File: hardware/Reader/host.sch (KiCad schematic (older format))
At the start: 7 parts

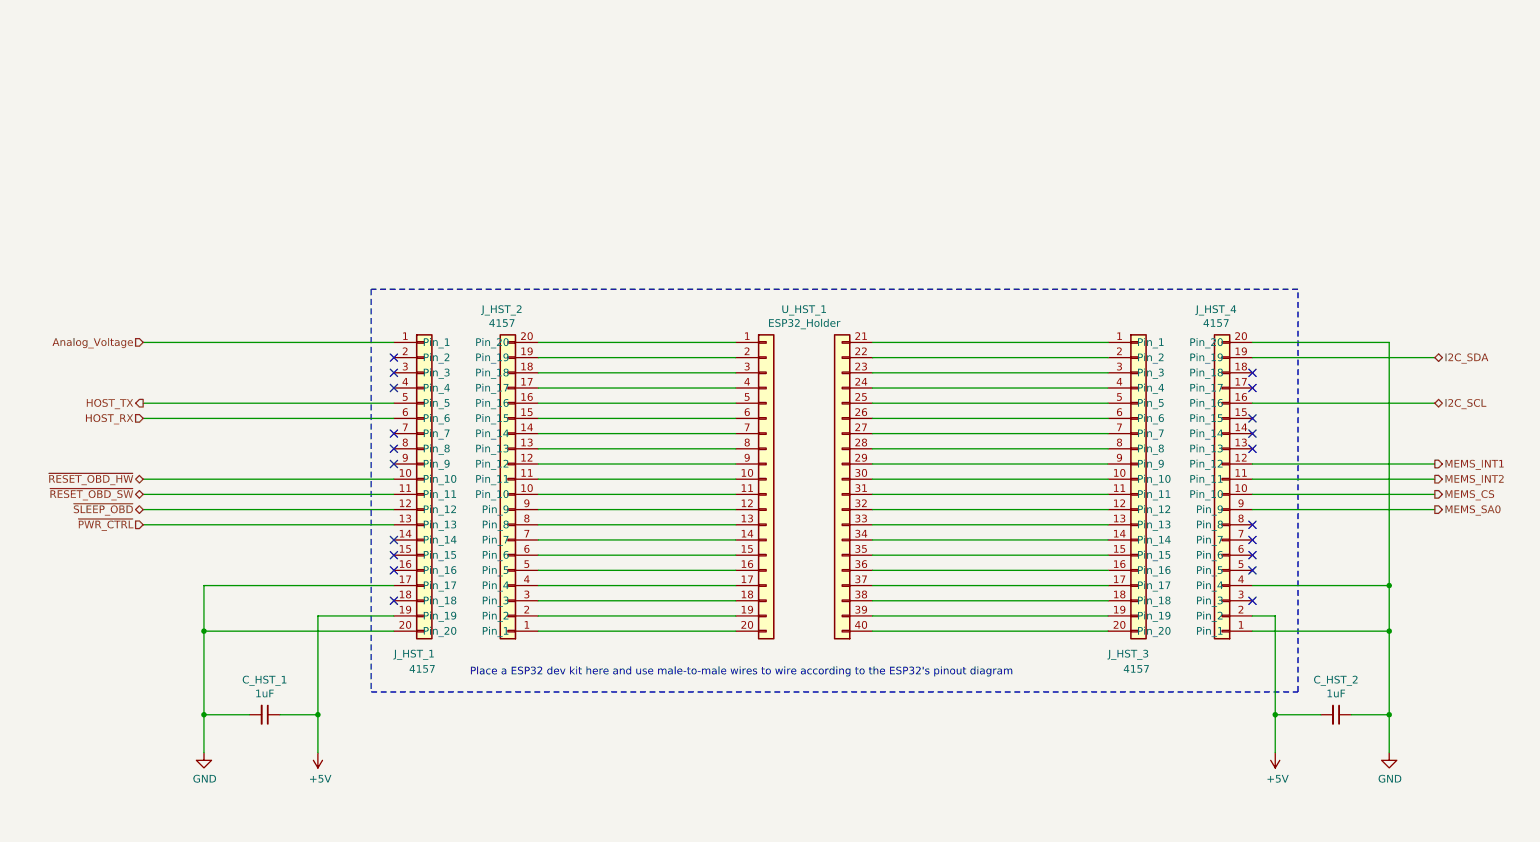
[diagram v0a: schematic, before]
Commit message: Revising reader
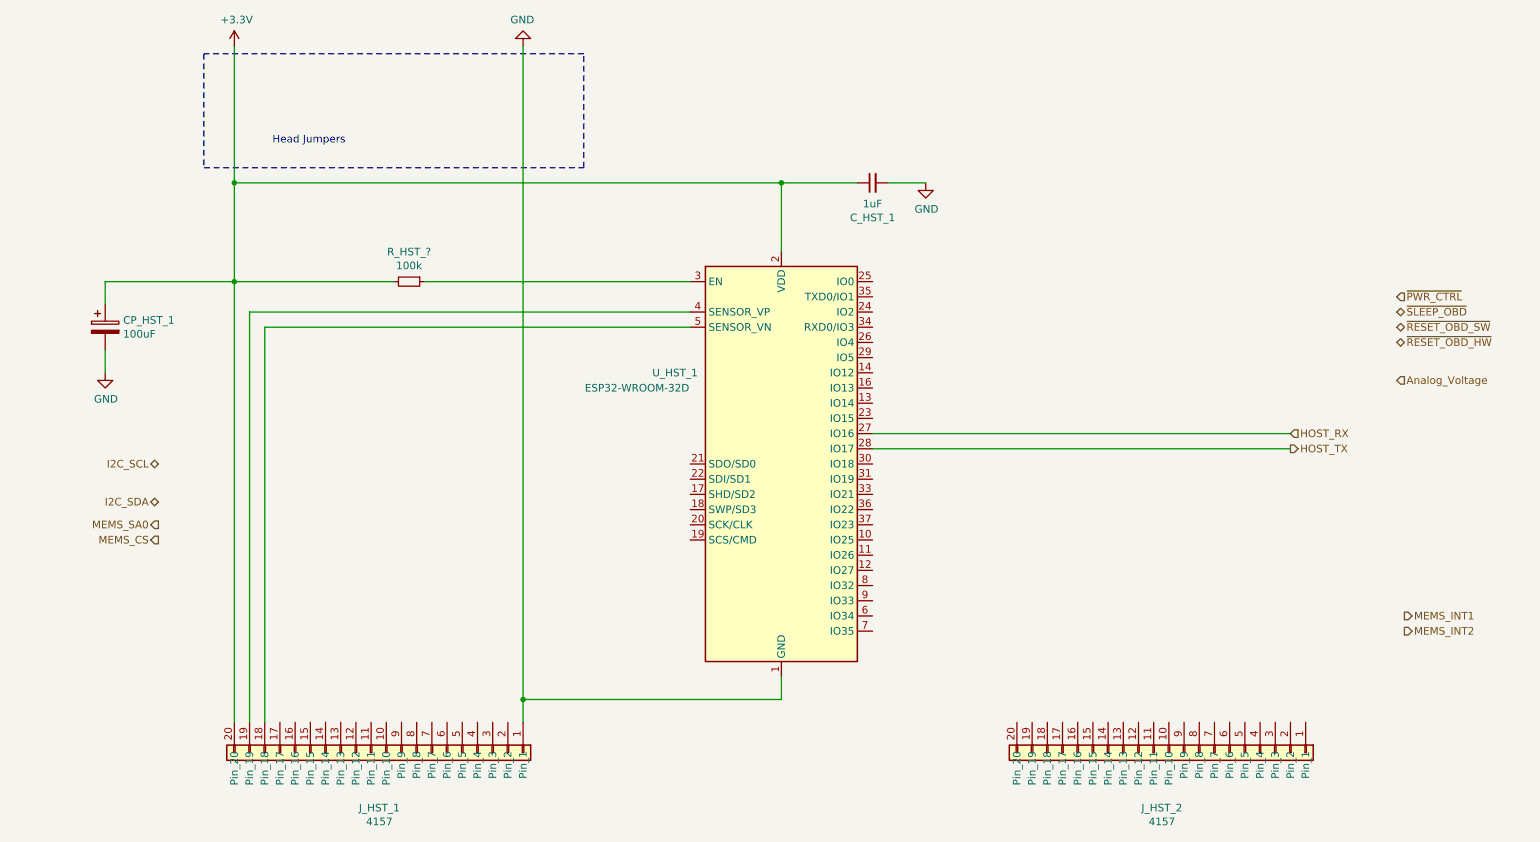
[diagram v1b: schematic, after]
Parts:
- removed C_HST_2: 1uF, footprints:0603, symbol Device:C_Small
- removed J_HST_3, J_HST_4: 4157, Connector_PinSocket_2.54mm:PinSocket_1x20_P2.54mm_Vertical, symbol CANtech:4157
- removed U_HST_1: ESP32_Holder, footprints:ESP32_Holder, symbol CANtech:ESP32_Holder
- added CP_HST_1: 100uF, symbol Device:CP
- added R_HST_?: 100k, footprints:RESC1608X55N, symbol Device:R_Small
- added U_HST_1: ESP32-WROOM-32D, RF_Module:ESP32-WROOM-32, symbol RF_Module:ESP32-WROOM-32D
- J_HST_1, J_HST_2: Part Name 4157 -> (none)
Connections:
- net Analog_Voltage: no longer J_HST_1.1 (Pin_1)
- net GND: now also J_HST_1.1 (Pin_1), CP_HST_1.2, U_HST_1.1 (GND), U_HST_1.15 (GND), U_HST_1.38 (GND), U_HST_1.39 (GND); no longer J_HST_1.17 (Pin_17), J_HST_1.20 (Pin_20)
- net HOST_RX: now also U_HST_1.27 (IO16); no longer J_HST_1.6 (Pin_6)
- net HOST_TX: now also U_HST_1.28 (IO17); no longer J_HST_1.5 (Pin_5)
- net ~PWR_CTRL~: no longer J_HST_1.13 (Pin_13)
- net ~RESET_OBD_HW~: no longer J_HST_1.10 (Pin_10)
- net ~RESET_OBD_SW~: no longer J_HST_1.11 (Pin_11)
- net ~SLEEP_OBD~: no longer J_HST_1.12 (Pin_12)
- net at J_HST_1.18 (Pin_18): now also U_HST_1.5 (SENSOR_VN)
- net +5V: no longer names the net of J_HST_1.19 (Pin_19)
- net +5V: now also U_HST_1.4 (SENSOR_VP); no longer C_HST_1.1
- new net: R_HST_?.1, U_HST_1.3 (EN)
- new net +3V3: CP_HST_1.1, C_HST_1.1, J_HST_1.20 (Pin_20), R_HST_?.2, U_HST_1.2 (VDD)
- no-connect marks 20 -> 0
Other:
- note added: "Head Jumpers"
- note removed: "Place a ESP32 dev kit here and use male-to-male wires to wire according to the ESP32's pinout diagram"
- moved on the sheet: C_HST_1
